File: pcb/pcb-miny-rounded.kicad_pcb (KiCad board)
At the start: 2 copper layers, 149.8 x 109.8 mm, 121 parts, among them J1 RP2040, J2 Conn_01x02_Socket, SW1 Switch, SW10 Switch, SW11 Switch, SW12 Switch, SW13 Switch, SW14 Switch, SW15 Switch, SW16 Switch, SW17 Switch, SW18 Switch, SW19 Switch, SW2 Switch, SW20 Switch, SW21 Switch, SW22 Switch, SW23 Switch, SW24 Switch, SW25 Switch, SW26 Switch, SW27 Switch, SW28 Switch, SW29 Switch, SW3 Switch, SW30 Switch, SW31 Switch, SW32 Switch, SW33 Switch, SW34 SW_SPDT, SW4 Switch, SW5 Switch, SW6 Switch, SW7 Switch, SW8 Switch, SW9 Switch

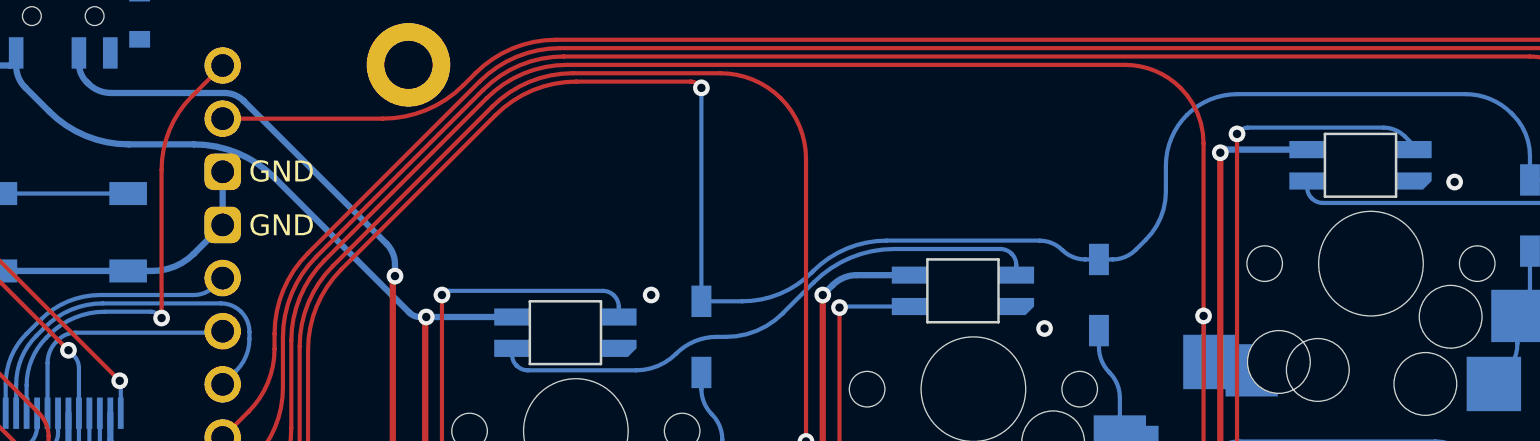
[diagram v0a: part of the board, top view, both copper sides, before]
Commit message: fix rounded pcb
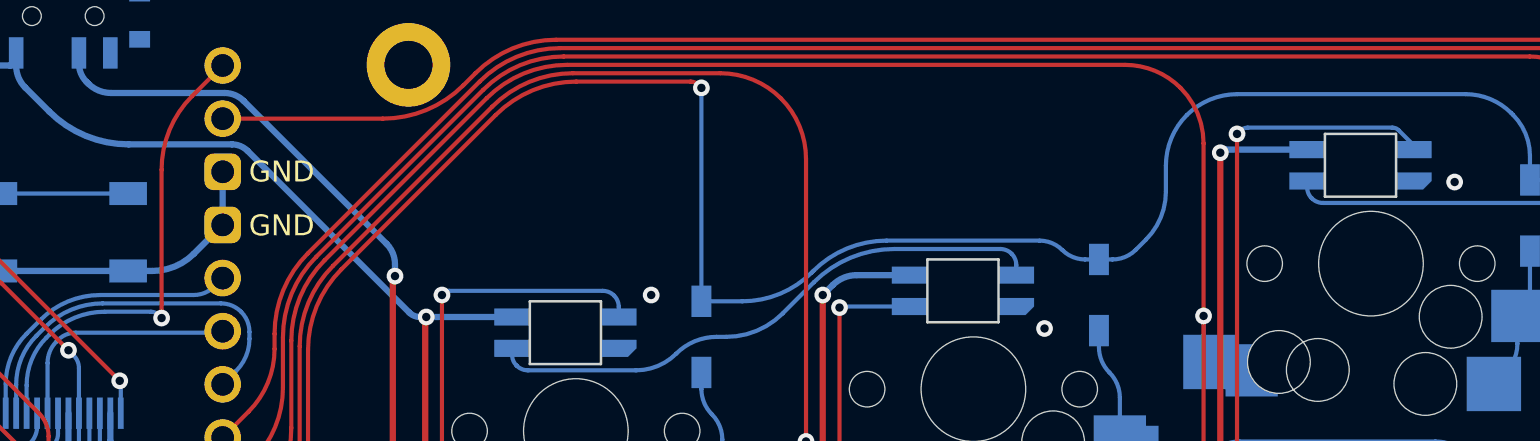
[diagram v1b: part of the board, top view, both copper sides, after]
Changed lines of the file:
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@@
 	)
 	(segment
-		(start 138.098105 82.499999)
+		(start 138.523511 82.499999)
 		(end 131.612985 82.499999)
 		(width 0.2)
@@
 	)
 	(segment
-		(start 139.12475 82.925249)
+		(start 138.823943 82.624442)
 		(end 139.479466 83.279965)
 		(width 0.2)
@@
 	)
 	(arc
-		(start 139.12475 82.925249)
-		(mid 138.653721 82.610517)
-		(end 138.098105 82.499999)
+		(start 138.823943 82.624442)
+		(mid 138.686104 82.532341)
+		(end 138.523511 82.499999)
 		(width 0.2)
 		(layer "B.Cu")
@@
 	)
 	(segment
-		(start 85.093792 84.893791)
+		(start 83.806647 83.606646)
 		(end 91.537867 91.337866)
 		(width 0.3)
@@
 	)
 	(segment
-		(start 81.246036 83.299999)
+		(start 83.066336 83.299999)
 		(end 78.127386 83.299999)
 		(width 0.3)
@@
 	)
 	(arc
-		(start 85.093792 84.893791)
-		(mid 83.328426 83.714212)
-		(end 81.246036 83.299999)
+		(start 83.806647 83.606646)
+		(mid 83.466989 83.379694)
+		(end 83.066336 83.299999)
 		(width 0.3)
 		(layer "B.Cu")
